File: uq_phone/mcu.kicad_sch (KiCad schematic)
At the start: 21 parts, among them J6 Conn_ARM_SWD_TagConnect_TC2030, U5 TXB0108RGYR, U6 TXB0108RGYR, U7 STM32H730VBTx

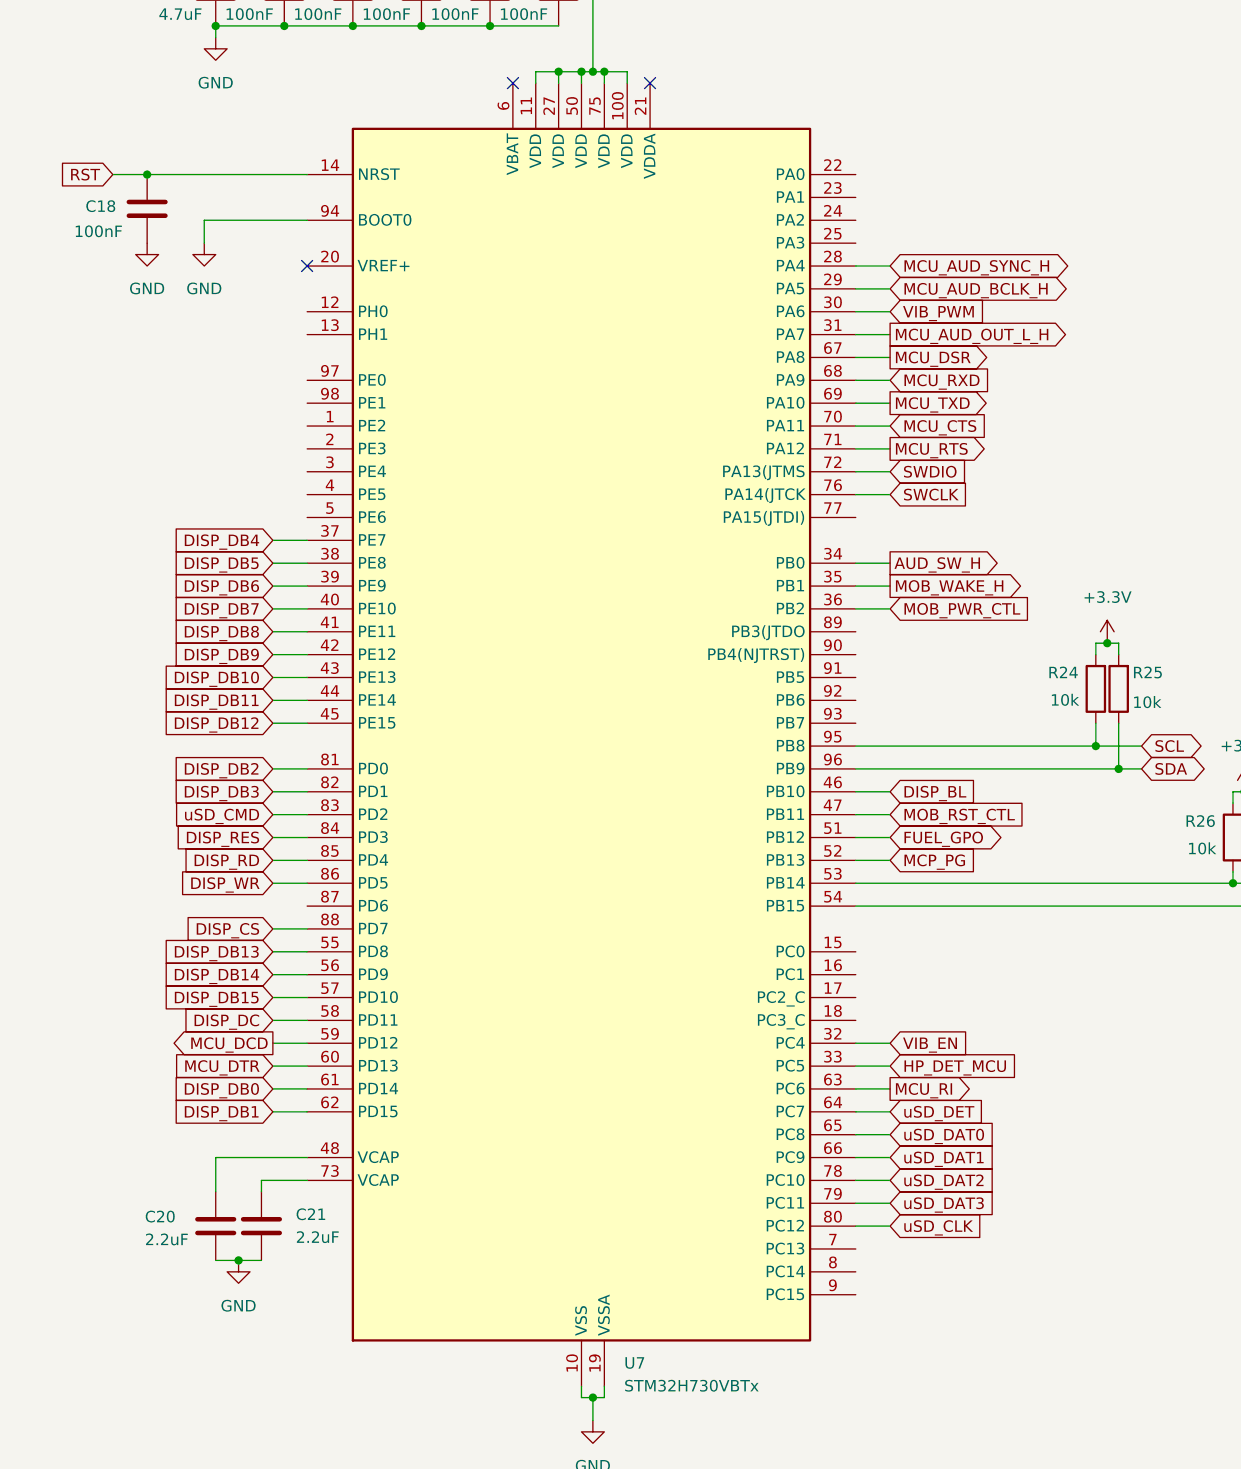
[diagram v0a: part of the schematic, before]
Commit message: Update Keypad
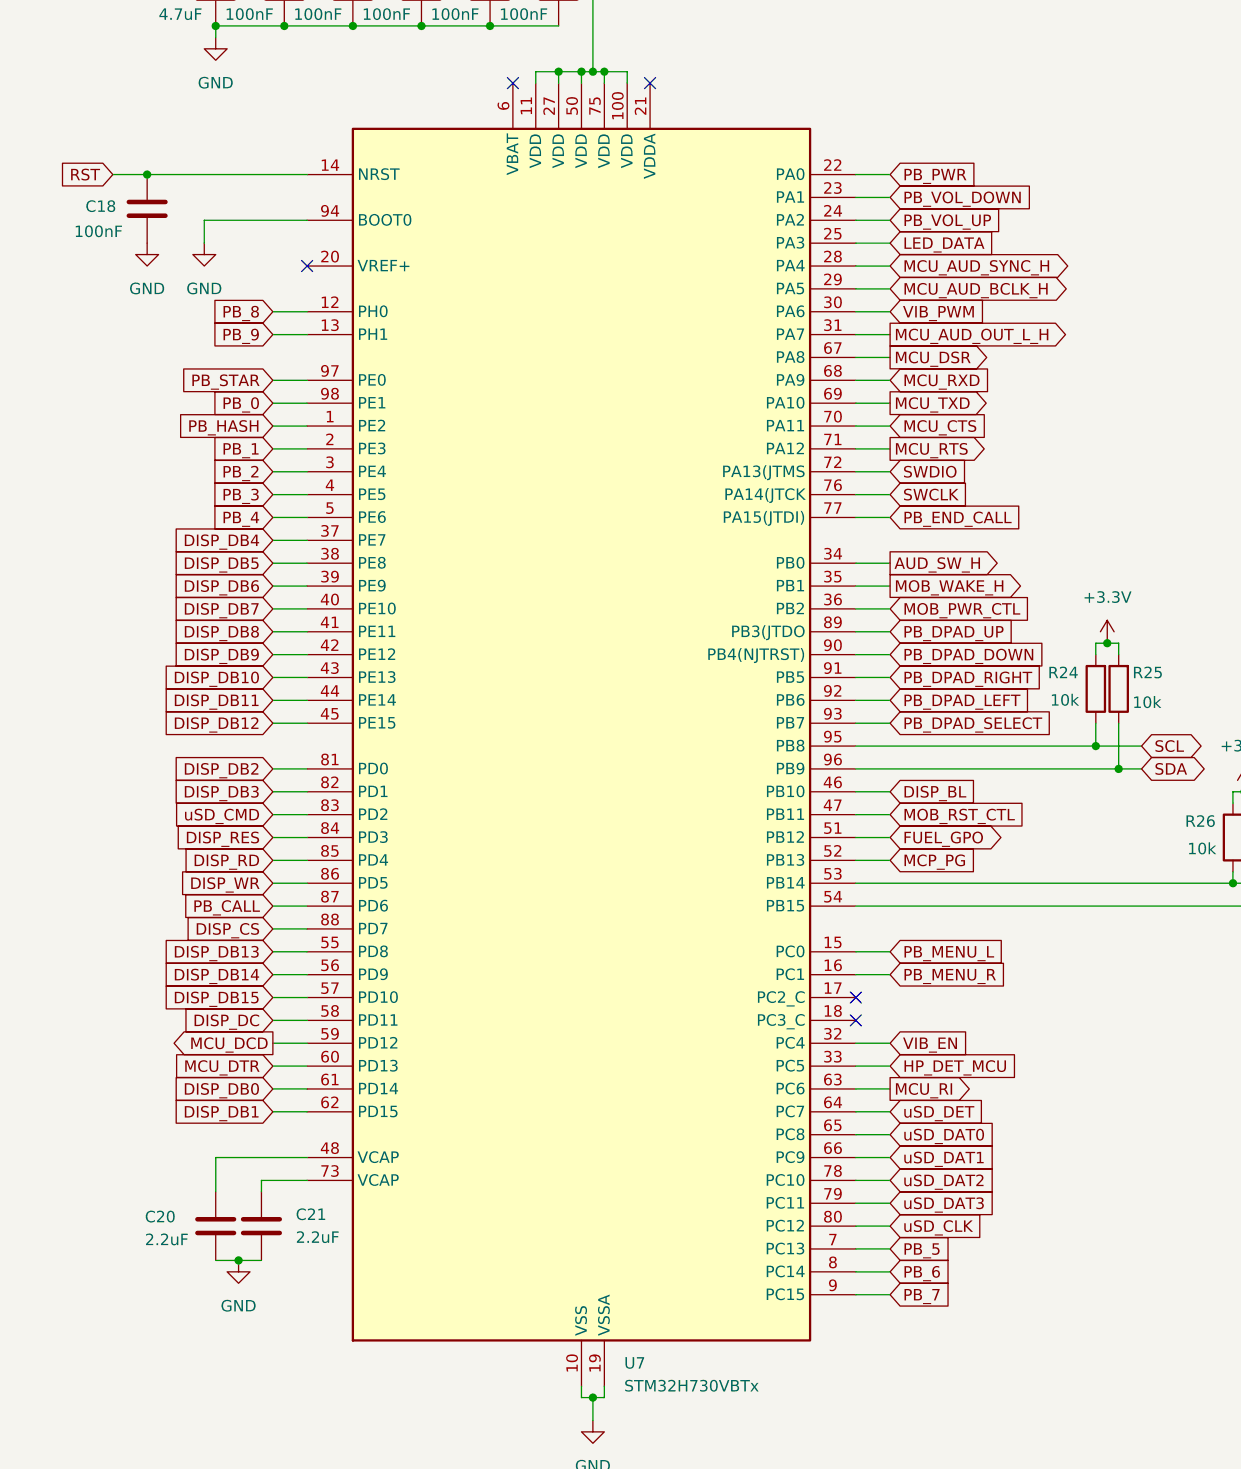
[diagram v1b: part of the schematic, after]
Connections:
- net PB_HASH: now reaches U7.1 (PE2)
- net PB_8: now reaches U7.12 (PH0)
- net PB_9: now reaches U7.13 (PH1)
- net PB_MENU_L: now reaches U7.15 (PC0)
- net PB_MENU_R: now reaches U7.16 (PC1)
- net PB_1: now reaches U7.2 (PE3)
- net PB_PWR: now reaches U7.22 (PA0)
- net PB_VOL_DOWN: now reaches U7.23 (PA1)
- net PB_VOL_UP: now reaches U7.24 (PA2)
- net LED_DATA: now reaches U7.25 (PA3)
- net PB_2: now reaches U7.3 (PE4)
- net PB_3: now reaches U7.4 (PE5)
- net PB_4: now reaches U7.5 (PE6)
- net PB_5: now reaches U7.7 (PC13)
- net PB_END_CALL: now reaches U7.77 (PA15(JTDI))
- net PB_6: now reaches U7.8 (PC14)
- net PB_CALL: now reaches U7.87 (PD6)
- net PB_DPAD_UP: now reaches U7.89 (PB3(JTDO)
- net PB_7: now reaches U7.9 (PC15)
- net PB_DPAD_DOWN: now reaches U7.90 (PB4(NJTRST))
- net PB_DPAD_RIGHT: now reaches U7.91 (PB5)
- net PB_DPAD_LEFT: now reaches U7.92 (PB6)
- net PB_DPAD_SELECT: now reaches U7.93 (PB7)
- net PB_STAR: now reaches U7.97 (PE0)
- net PB_0: now reaches U7.98 (PE1)
- no-connect marks 4 -> 6
